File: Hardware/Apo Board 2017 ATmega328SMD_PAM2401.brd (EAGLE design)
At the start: 85.1 x 52.7 mm, 38 parts, among them Q1 RESONATORSMD, U1 LED-TRICOLOR-5050-IC, U10 LED-TRICOLOR-5050-IC, U11 LED-TRICOLOR-5050-IC, U13 ATMEGA328, U2 PAM2401, U3 LED-TRICOLOR-5050-IC, U4 LED-TRICOLOR-5050-IC, U5 LED-TRICOLOR-5050-IC, U6 LED-TRICOLOR-5050-IC, U7 LED-TRICOLOR-5050-IC, U8 LED-TRICOLOR-5050-IC, U9 LED-TRICOLOR-5050-IC

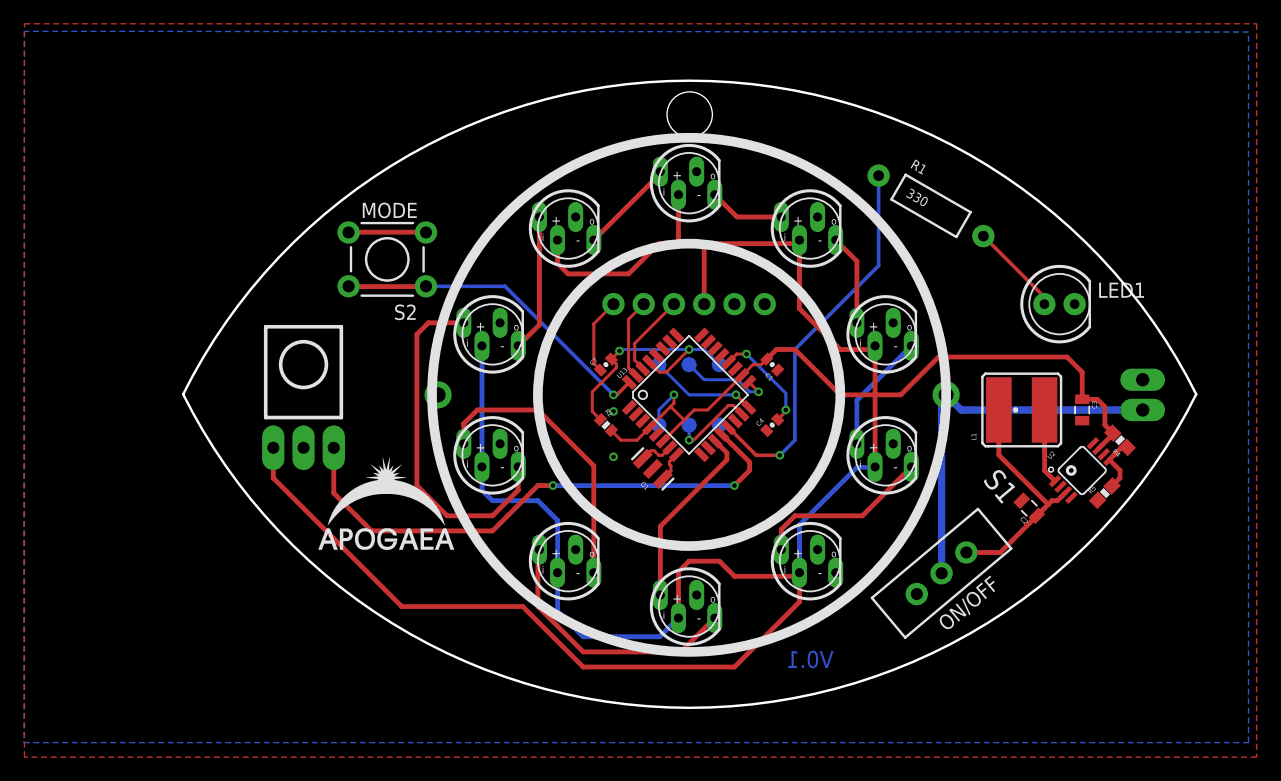
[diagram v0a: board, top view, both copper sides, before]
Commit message: Final touches before review
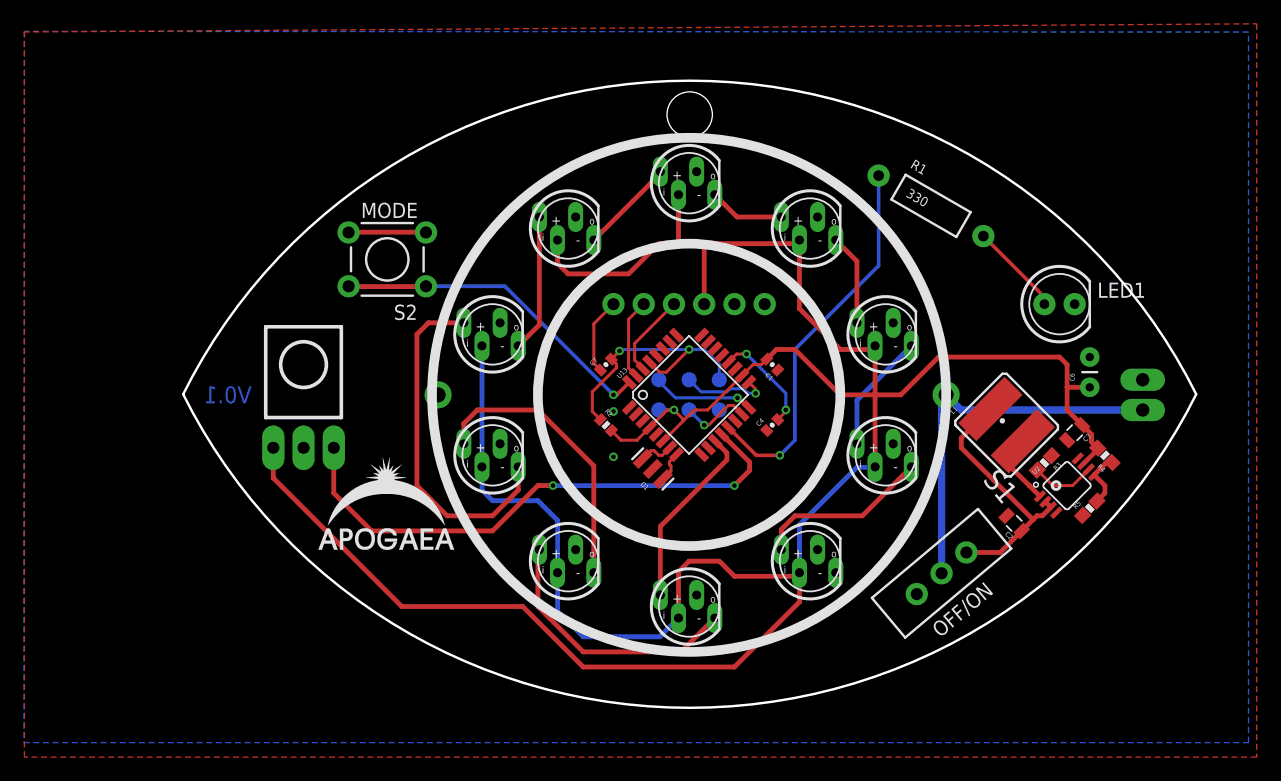
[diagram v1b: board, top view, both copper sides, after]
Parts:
- added C6: (no value), SparkFun-Capacitors:CAP-PTH-SMALL
- added R3: 100k, SparkFun-Resistors:0603-RES
- moved C3 2.01 mm to (32.4, -3.17), turned to 225 degrees
- moved U2 1.80 mm to (31.8, -7.62)
- moved R4 1.80 mm to (34.9, -5.08)
- moved L1 1.80 mm to (26.7, -2.54), turned to 45 degrees
- moved C2 1.80 mm to (27.3, -10.8)
- moved R5 1.80 mm to (33.7, -9.53)
- moved TP1 1.27 mm to (-2.54, -1.27)
- moved TP2 1.27 mm to (0.00, -1.27)
- moved TP3 1.27 mm to (2.54, -1.27)
- moved TP4 1.27 mm to (-2.54, 1.27)
- moved TP5 1.27 mm to (0.00, 1.27)
- moved TP6 1.27 mm to (2.54, 1.27)
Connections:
- new net N$4: R3.2, U2.6
- net +5V: now also C6.1
- net GND: now also C6.2, R3.1
- net N$10: now also U2.2
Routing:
- net N$4: track 0.00 -> 5.43 mm
- net N$10: track 20.1 -> 22.1 mm
- net +5V: track 254.6 -> 253.0 mm
- net MOSI: track 7.23 -> 5.96 mm
- net RESET: track 20.8 -> 22.0 mm
- net SCK: track 7.95 -> 7.44 mm
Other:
- board text added: "3)Press button to share mode"
- board text added: "4)Collect as many modes as you can"
- board text added: "5V"
- board text added: "GND"
- board text added: "How to Play: 1)Two Eyeballs see one another 2)LEDs start pulsing"
- board text added: "MISO"
- board text added: "MOSI"
- board text added: "OFF/ON"
- board text added: "RST"
- board text added: "SCK"
- board text added: "SOLDER ON THIS SIDE"
- board text removed: "ON/OFF"

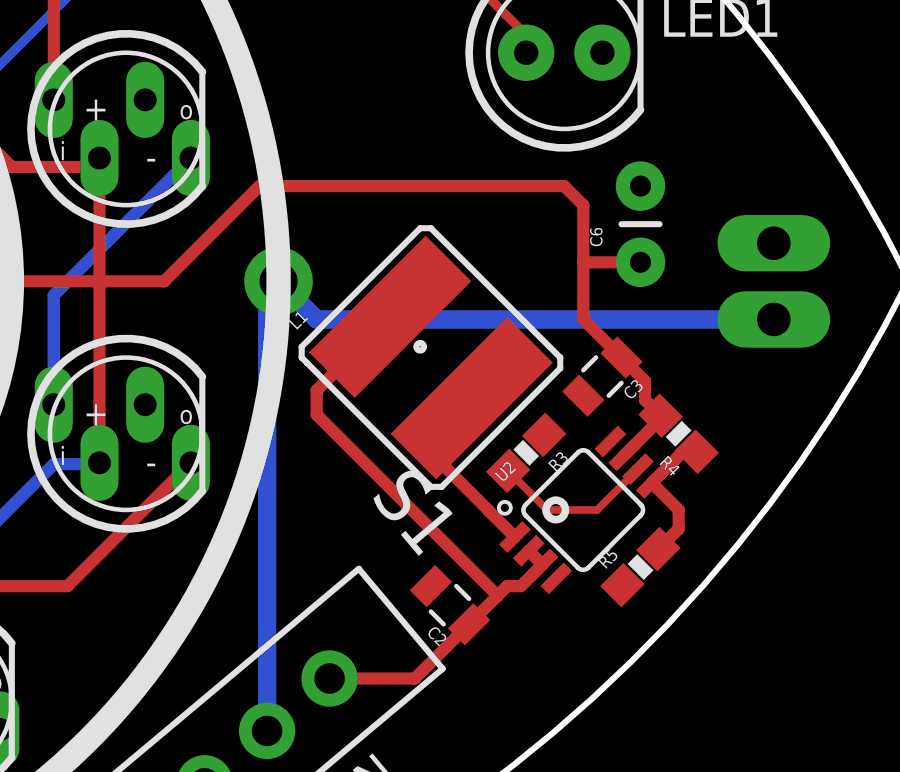
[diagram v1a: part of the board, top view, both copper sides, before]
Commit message: Fixing Natural Jumper and few moonier text tweaks
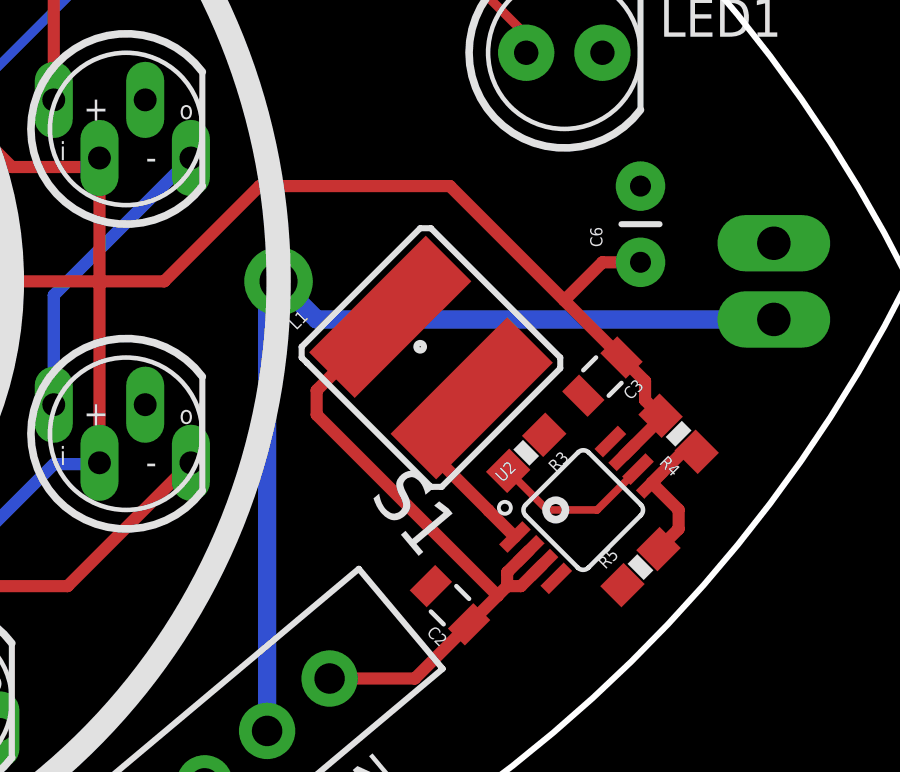
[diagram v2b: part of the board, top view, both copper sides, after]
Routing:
- net +5V: track 253.0 -> 252.0 mm
- net N$10: track 22.1 -> 23.0 mm
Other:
- board text added: "BLK-"
- board text added: "RED+"
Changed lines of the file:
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@@
 <?xml version="1.0" encoding="utf-8"?>
 <!DOCTYPE eagle SYSTEM "eagle.dtd">
-<eagle version="7.3.0">
+<eagle version="7.6.0">
 <drawing>
 <settings>
@@
 <layer number="20" name="Dimension" color="15" fill="1" visible="yes" active="yes"/>
 <layer number="21" name="tPlace" color="16" fill="1" visible="yes" active="yes"/>
-<layer number="22" name="bPlace" color="14" fill="1" visible="no" active="yes"/>
+<layer number="22" name="bPlace" color="14" fill="1" visible="yes" active="yes"/>
 <layer number="23" name="tOrigins" color="15" fill="1" visible="yes" active="yes"/>
-<layer number="24" name="bOrigins" color="15" fill="1" visible="no" active="yes"/>
-<layer number="25" name="tNames" color="7" fill="1" visible="yes" active="yes"/>
+<layer number="24" name="bOrigins" color="15" fill="1" visible="yes" active="yes"/>
+<layer number="25" name="tNames" color="7" fill="1" visible="no" active="yes"/>
 <layer number="26" name="bNames" color="7" fill="1" visible="no" active="yes"/>
 <layer number="27" name="tValues" color="7" fill="1" visible="no" active="yes"/>
@@
 <layer number="43" name="vRestrict" color="2" fill="10" visible="no" active="yes"/>
 <layer number="44" name="Drills" color="7" fill="1" visible="no" active="yes"/>
-<layer number="45" name="Holes" color="7" fill="1" visible="no" active="yes"/>
+<layer number="45" name="Holes" color="7" fill="1" visible="yes" active="yes"/>
 <layer number="46" name="Milling" color="3" fill="1" visible="no" active="yes"/>
 <layer number="47" name="Measures" color="7" fill="1" visible="no" active="yes"/>
 <layer number="48" name="Document" color="7" fill="1" visible="no" active="yes"/>
-<layer number="49" name="Reference" color="13" fill="1" visible="no" active="yes"/>
+<layer number="49" name="Reference" color="13" fill="1" visible="yes" active="yes"/>
 <layer number="50" name="dxf" color="7" fill="1" visible="no" active="yes"/>
-<layer number="51" name="tDocu" color="6" fill="1" visible="no" active="yes"/>
+<layer number="51" name="tDocu" color="6" fill="1" visible="yes" active="yes"/>
 <layer number="52" name="bDocu" color="7" fill="1" visible="no" active="yes"/>
 <layer number="53" name="tGND_GNDA" color="7" fill="9" visible="no" active="no"/>
@@
 <text x="-13.843" y="-13.97" size="0.9398" layer="22" font="vector" ratio="15" rot="MR0">3)Press button to
 share mode</text>
+<text x="39.37" y="-3.81" size="1.016" layer="22" font="vector" ratio="15" rot="MR0">RED+</text>
+<text x="39.37" y="2.54" size="1.016" layer="22" font="vector" ratio="15" rot="MR0">BLK-</text>
 </plain>
 <attributes>
@@
 <wire x1="9.271" y1="-17.399" x2="9.271" y2="-14.9384" width="0.4064" layer="1"/>
 <contactref element="C6" pad="1"/>
-<wire x1="31.115" y1="3.175" x2="20.955" y2="3.175" width="0.4064" layer="1"/>
-<wire x1="31.115" y1="3.175" x2="31.75" y2="2.54" width="0.4064" layer="1"/>
-<wire x1="31.75" y1="2.54" x2="31.75" y2="0.635" width="0.4064" layer="1"/>
-<wire x1="33.655" y1="0.635" x2="31.75" y2="0.635" width="0.4064" layer="1"/>
 <wire x1="34.32395625" y1="-4.47895625" x2="33.8074" y2="-3.9624" width="0.4064" layer="1"/>
 <wire x1="33.8074" y1="-3.9624" x2="33.8074" y2="-3.324609375" width="0.4064" layer="1"/>
 <wire x1="33.8074" y1="-3.324609375" x2="33.02139375" y2="-2.538603125" width="0.4064" layer="1"/>
 <wire x1="33.02139375" y1="-2.538603125" x2="33.018603125" y2="-2.538603125" width="0.4064" layer="1"/>
-<wire x1="33.018603125" y1="-2.538603125" x2="31.75" y2="-1.27" width="0.4064" layer="1"/>
-<wire x1="31.75" y1="-1.27" x2="31.75" y2="0.635" width="0.4064" layer="1"/>
 <wire x1="-3.31816875" y1="-2.75248125" x2="-1.8356875" y2="-1.27" width="0.254" layer="1"/>
 <wire x1="-1.8356875" y1="-1.27" x2="-1.27" y2="-1.27" width="0.254" layer="1"/>
@@
 <wire x1="34.32395625" y1="-4.586421875" x2="34.323959375" y2="-4.58641875" width="0.3048" layer="1"/>
 <wire x1="34.323959375" y1="-4.58641875" x2="34.32395625" y2="-4.47895625" width="0.3048" layer="1"/>
+<wire x1="33.018603125" y1="-2.538603125" x2="31.115" y2="-0.635" width="0.4064" layer="1"/>
+<wire x1="31.115" y1="-0.635" x2="27.305" y2="3.175" width="0.4064" layer="1"/>
+<wire x1="27.305" y1="3.175" x2="20.955" y2="3.175" width="0.4064" layer="1"/>
+<wire x1="33.655" y1="0.635" x2="32.385" y2="0.635" width="0.4064" layer="1"/>
+<wire x1="32.385" y1="0.635" x2="31.115" y2="-0.635" width="0.4064" layer="1"/>
 </signal>
 <signal name="TX">
@@
 <contactref element="U2" pad="2"/>
 <wire x1="28.8925" y1="-10.4775" x2="27.94139375" y2="-11.42860625" width="0.4064" layer="1"/>
-<wire x1="29.9292" y1="-8.981178125" x2="30.38881875" y2="-9.440796875" width="0.4064" layer="1"/>
 <wire x1="22.86" y1="-4.445" x2="22.86" y2="-3.63470625" width="0.4064" layer="1"/>
 <wire x1="22.86" y1="-3.63470625" x2="25.312353125" y2="-1.182353125" width="0.4064" layer="1"/>
 <wire x1="27.94139375" y1="-11.43139375" x2="27.94139375" y2="-11.42860625" width="0.3048" layer="1"/>
+<wire x1="29.9292" y1="-8.981178125" x2="29.21" y2="-9.700378125" width="0.4064" layer="1"/>
+<wire x1="29.21" y1="-9.700378125" x2="29.21" y2="-10.16" width="0.4064" layer="1"/>
 </signal>
 <signal name="N$12">

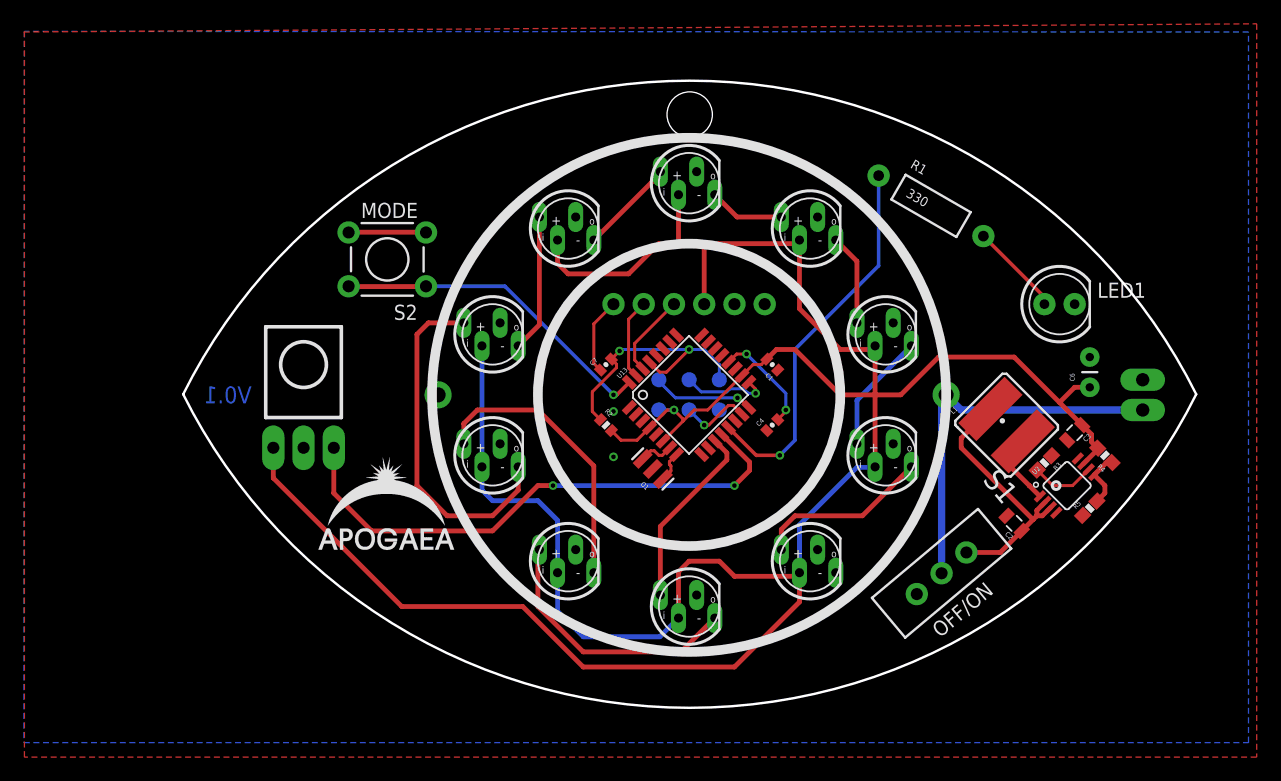
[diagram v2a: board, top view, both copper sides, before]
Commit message: Final version for Prototypes V0.1 and GERBERS
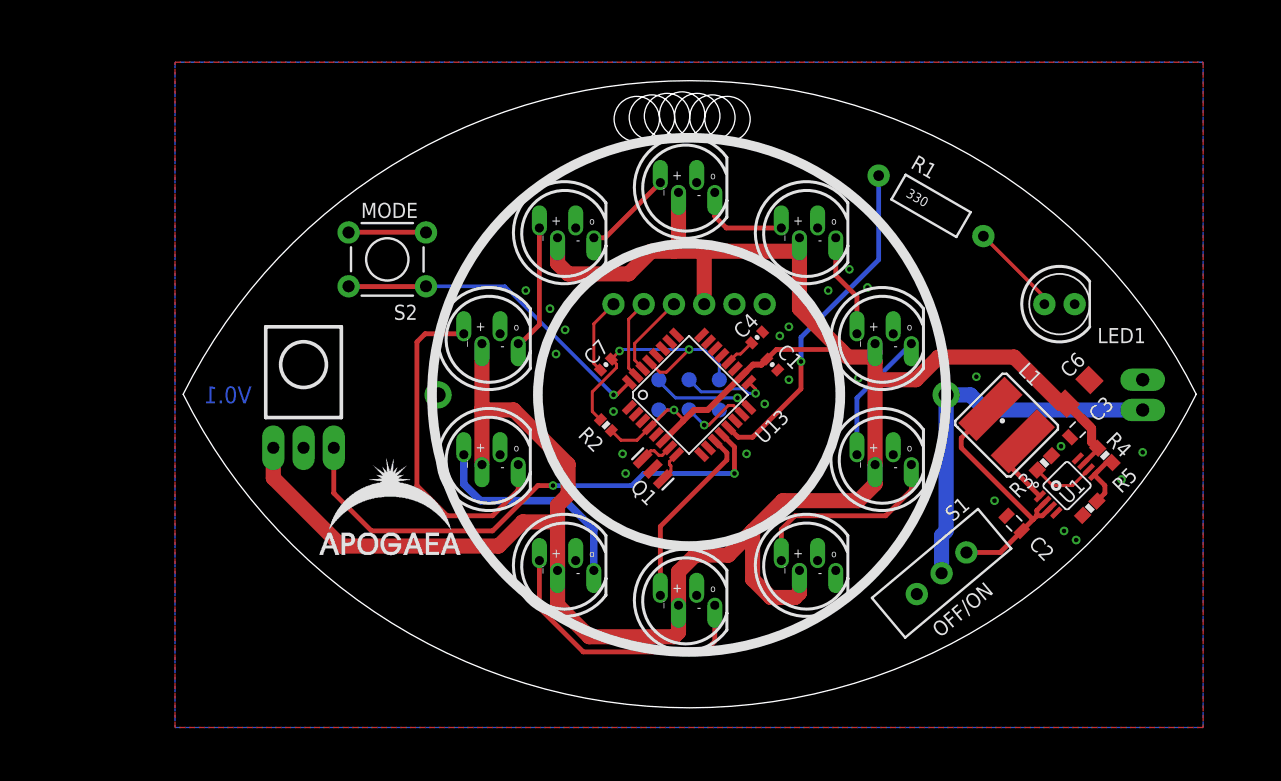
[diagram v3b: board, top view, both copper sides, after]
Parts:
- added U$1, U$2: (no value), Openponics:APOLOGO
- C6: device SparkFun-Capacitors:CAP-PTH-SMALL -> SparkFun-Capacitors:1206
- U1: value LED-TRICOLOR-5050-IC -> PAM2401; device SparkFun-LED:LED-RGB-THRU -> SparkFun-PowerIC:MSOP8
- U2: value PAM2401 -> LED-TRICOLOR-5050-IC; device SparkFun-PowerIC:MSOP8 -> SparkFun-LED:LED-RGB-THRU
- moved U1 15.5 mm to (31.8, -7.62), turned to 315 degrees
- moved U2 15.5 mm to (16.5, -5.08), turned to 180 degrees
- moved C4 7.47 mm to (5.71, 4.83), turned to 225 degrees
- moved C6 1.09 mm to (32.6, 0.25), turned to 45 degrees
- moved U7 0.89 mm to (0.00, -16.9)
- moved C3 0.36 mm to (32.6, -2.92)
- renumbered JP1 to U12
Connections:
- net N$7 renamed +BATT_RAW
- net +5V: now also U1.7, U2.2; no longer U1.2, U2.7
- net GND: now also U1.4, U1.8, U2.3; no longer U1.3, U2.4, U2.8
- net N$10: now also U1.2, U1.3; no longer U2.2, U2.3
- net N$12: now also U1.5; no longer U2.5
- net N$13: now also U2.1; no longer U1.1
- net N$14: now also U2.4; no longer U1.4
- net N$4: now also U1.6; no longer U2.6
- net N$8: now also U1.1; no longer U2.1
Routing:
- net +5V: track 252.0 -> 219.1 mm
- net AREF: track 8.95 -> 2.61 mm, vias 2 -> 0
- net N$2: track 24.0 -> 18.4 mm
- net IR_TX: track 32.2 -> 28.7 mm
- net N$14: track 14.8 -> 17.1 mm
- net IR_RX: track 46.2 -> 44.5 mm
- net N$9: track 6.36 -> 8.01 mm
- net N$1: track 22.4 -> 23.6 mm
- net N$13: track 10.1 -> 11.2 mm
- net N$11: track 7.69 -> 8.80 mm
- net N$6: track 11.6 -> 10.6 mm
- net N$5: track 29.4 -> 28.9 mm
- net DOUT_DIN: track 8.06 -> 7.51 mm
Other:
- board text added: "3) Press button to share mode"
- board text added: "4) Collect as many modes as you can"
- board text added: "How to Play: 1) Two Eyeballs see one another 2) LEDs start pulsing"
- board text removed: "3)Press button to share mode"
- board text removed: "4)Collect as many modes as you can"
- board text removed: "How to Play: 1)Two Eyeballs see one another 2)LEDs start pulsing"
